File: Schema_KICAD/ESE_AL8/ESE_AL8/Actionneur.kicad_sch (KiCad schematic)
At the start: 15 parts, among them J8 ECRAN, U4 ZXBM5210-SP, U5 ZXBM5210-SP

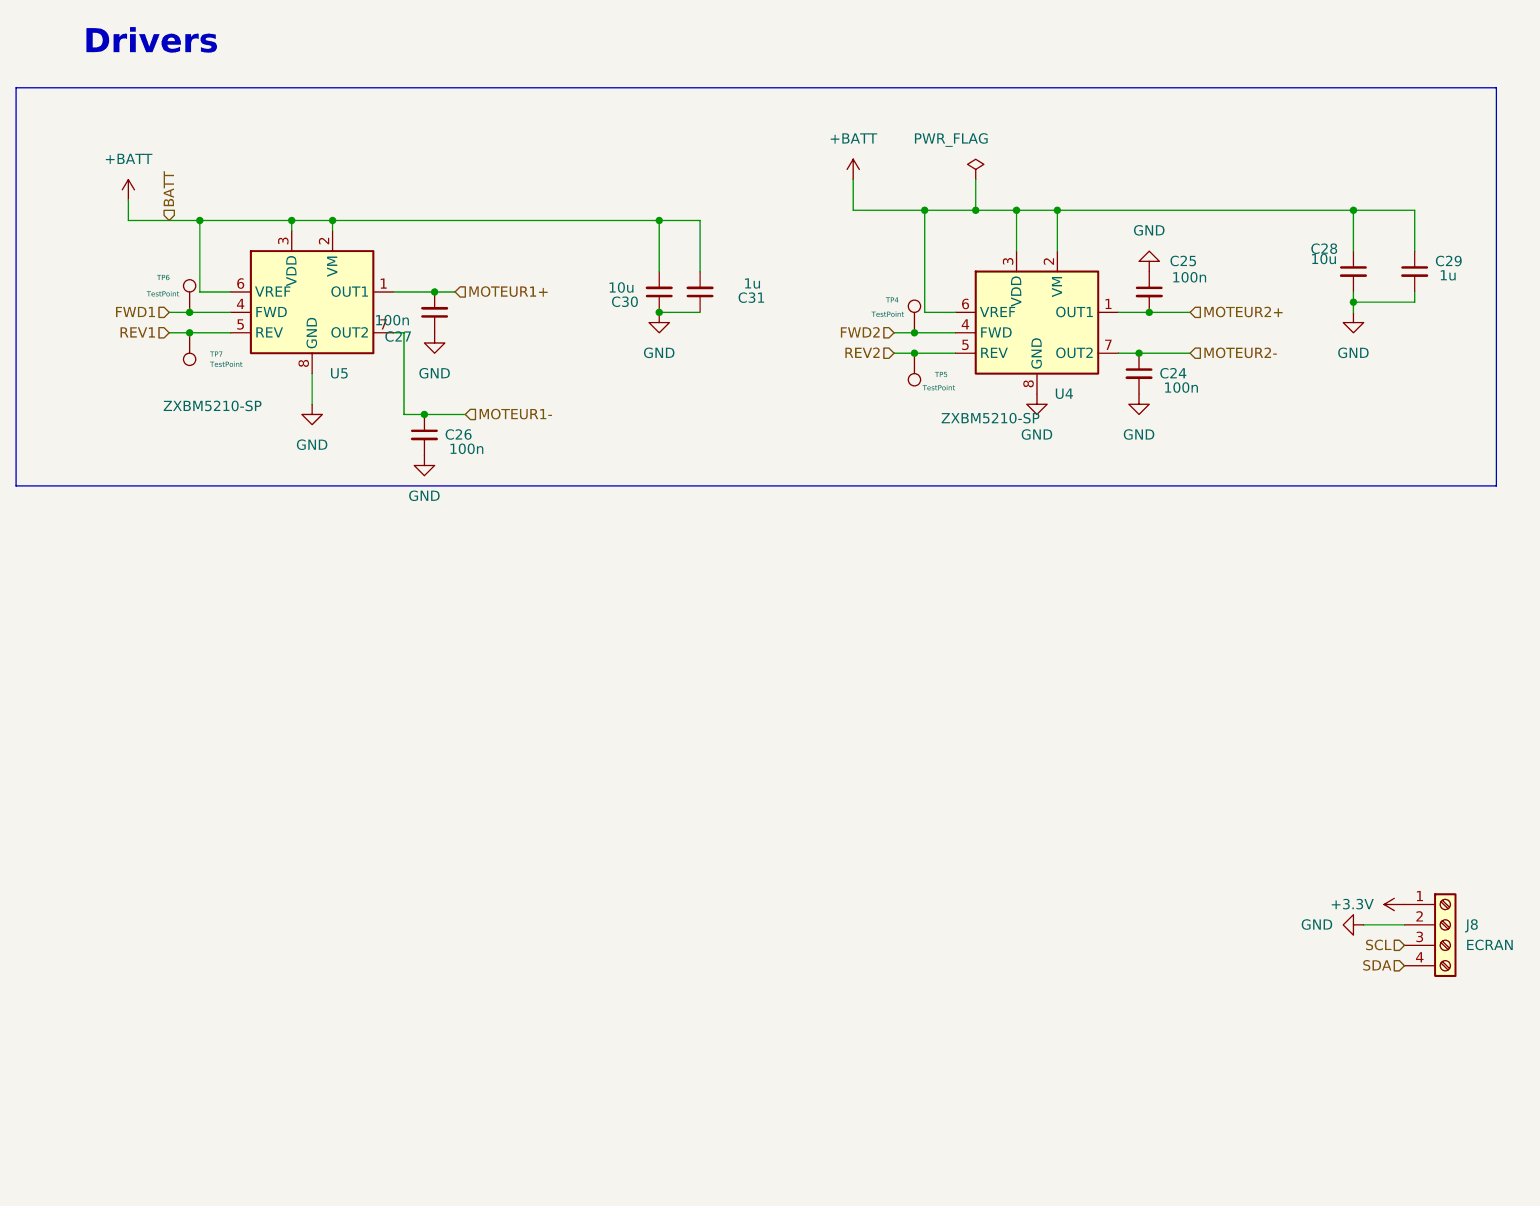
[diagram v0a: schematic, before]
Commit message: new version
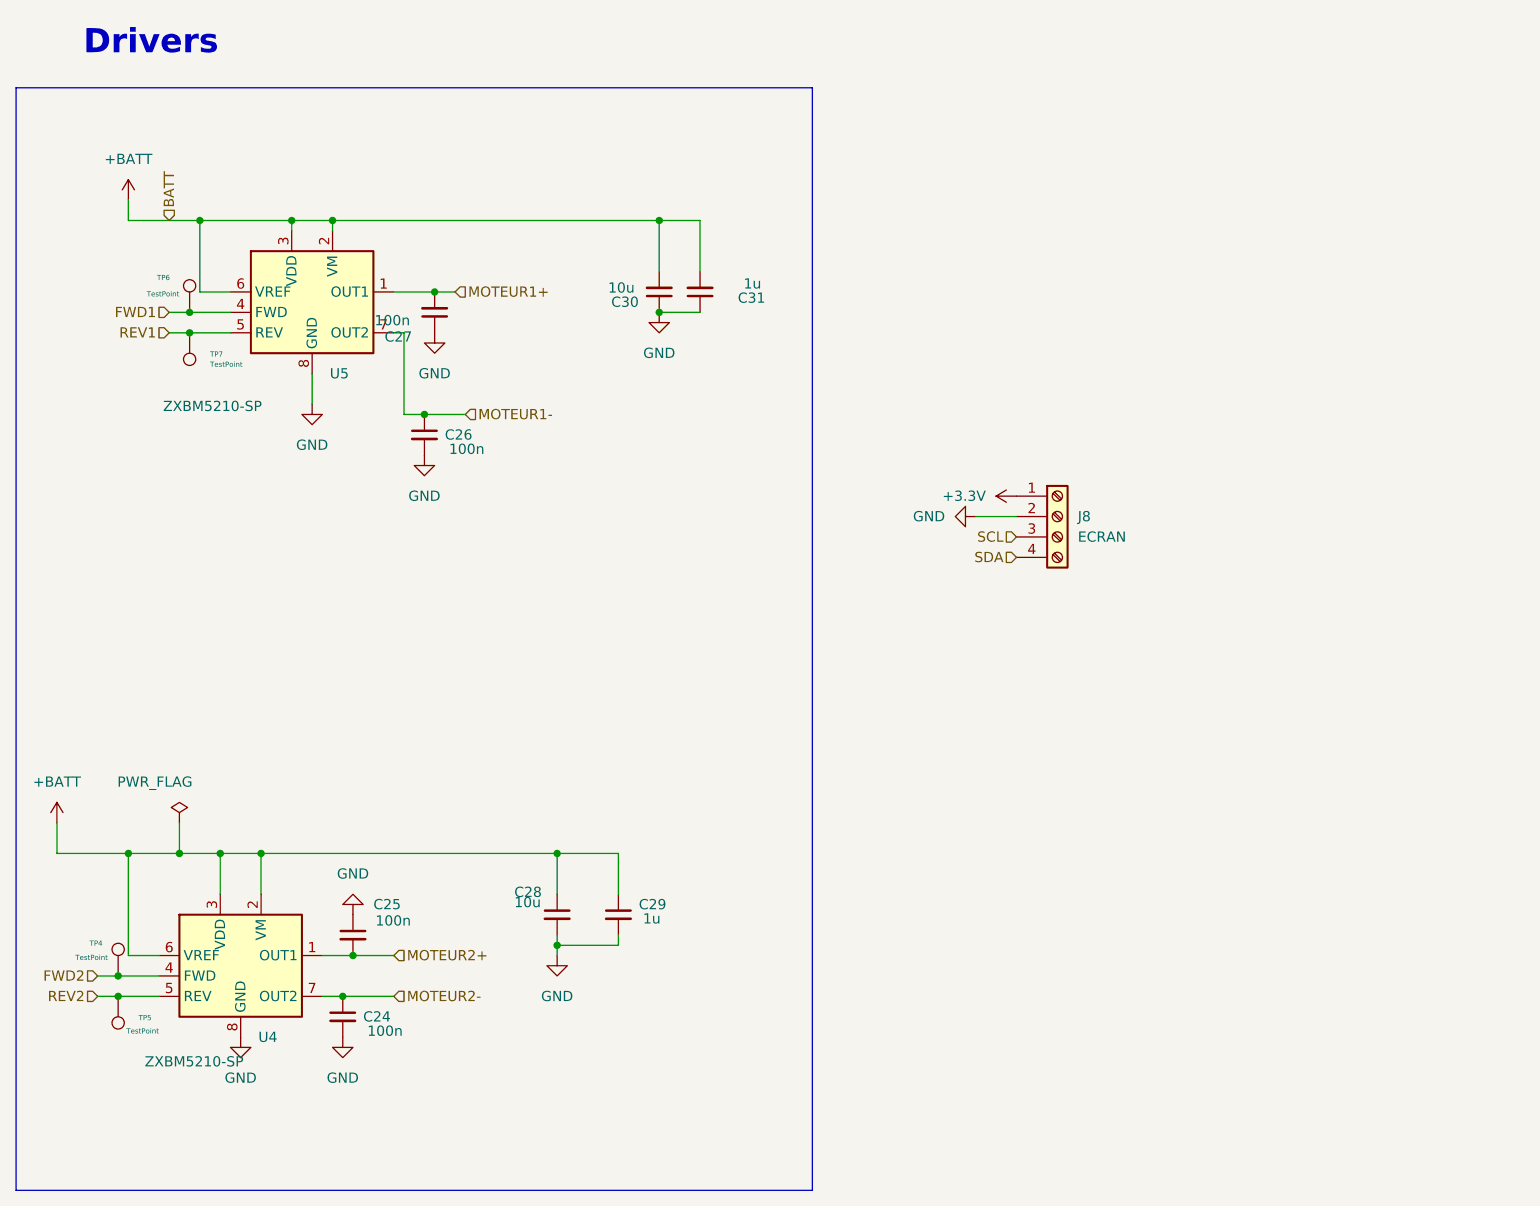
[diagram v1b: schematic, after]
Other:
- moved on the sheet: J8

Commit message: commit
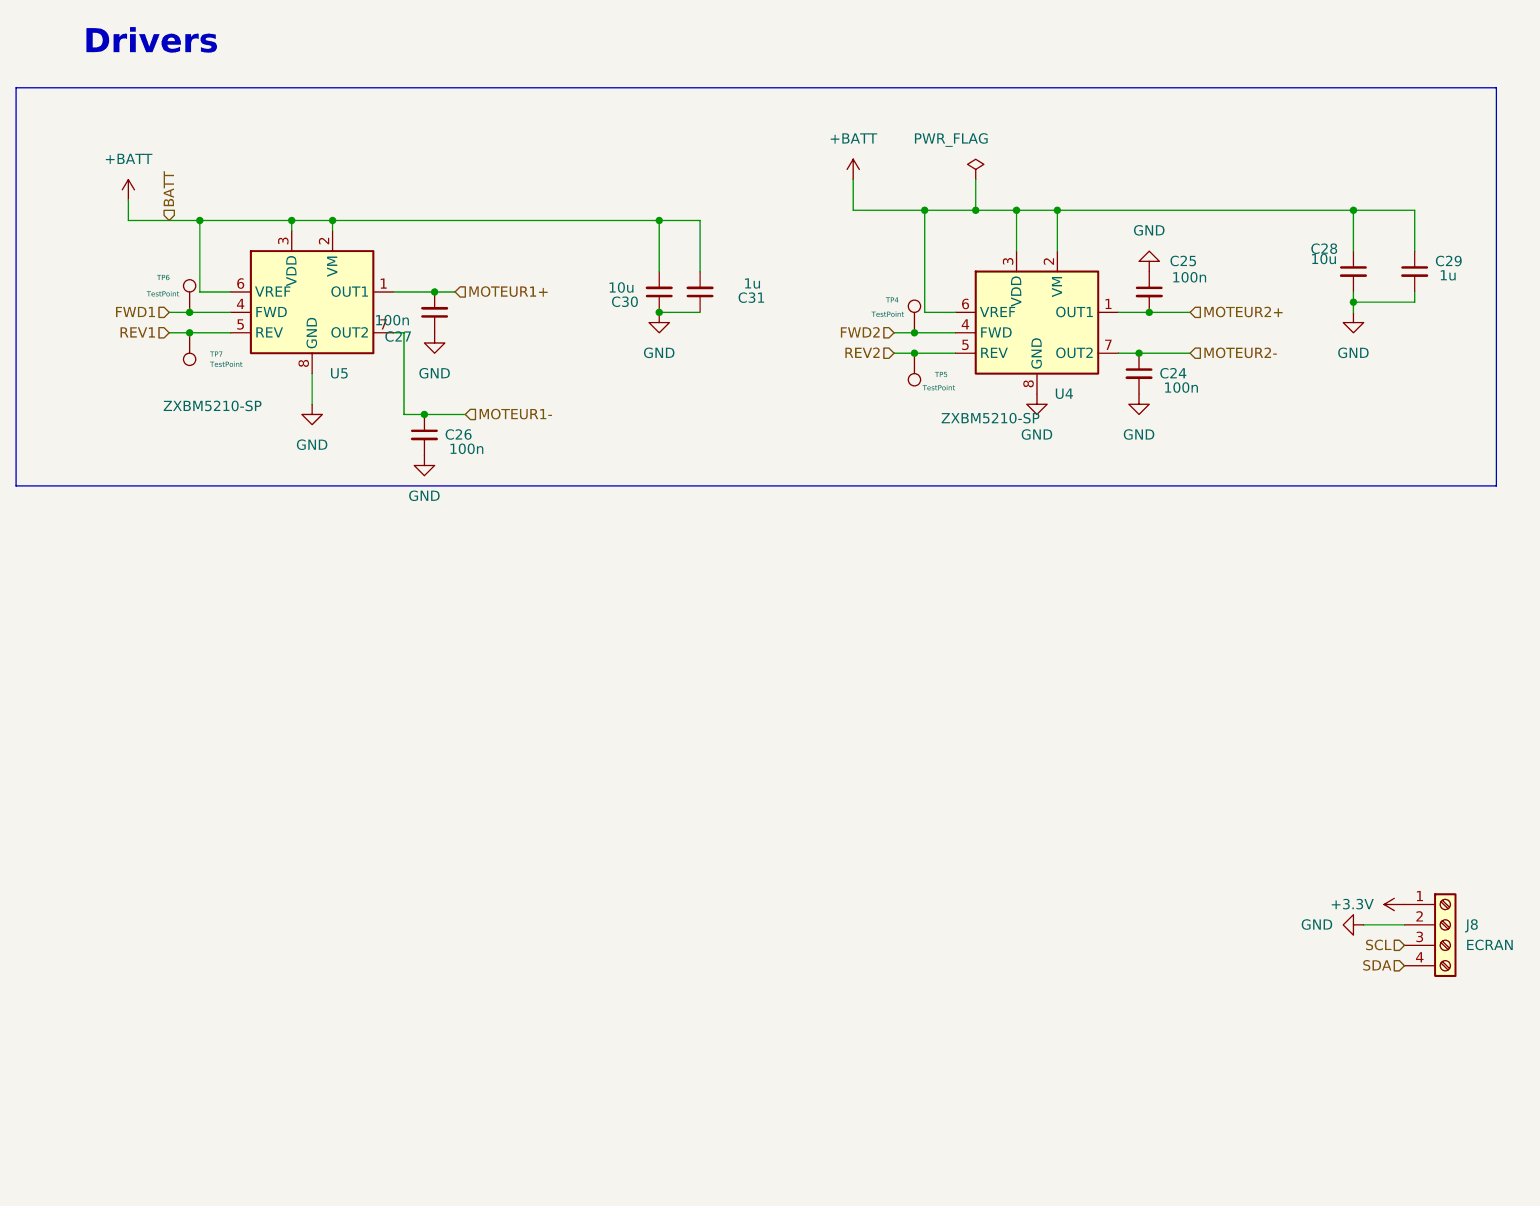
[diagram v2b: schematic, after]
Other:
- moved on the sheet: J8
